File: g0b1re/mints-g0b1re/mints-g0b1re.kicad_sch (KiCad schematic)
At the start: 34 parts, among them J1 Conn_01x08, J3 Conn_01x02, J4 Conn_01x04, J5 Conn_01x04, J6 FTSH-107-01-X-DV-K, J7 Conn_01x04, SW1 SW_Coded_SH-7050, U1 STM32G0B1RETx, U2 TCAN3414DDFR, U5 AP63203WU

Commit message: polishing schematic, add variants, fix some small issues
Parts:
- removed J7: Conn_01x04, Connector_PinHeader_2.54mm:PinHeader_1x04_P2.54mm_Vertical, symbol Connector_Generic:Conn_01x04
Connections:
- net CAN+: now also J4.2 (Pin_2); no longer J5.1 (Pin_1)
- net CAN-: now also J4.3 (Pin_3); no longer J5.4 (Pin_4)
- net GND: now also J4.4 (Pin_4), J5.4 (Pin_4); no longer J4.1 (Pin_1), J4.2 (Pin_2)
- net SPI_nCS: now reaches U1.36 (PA8)
- net CANRX renamed CAN_RXD
- net CAN_RXD: now also U1.25 (PC4); no longer U1.26 (PC5)
- net CANTX renamed CAN_TXD
- net CAN_TXD: now also U1.26 (PC5); no longer U1.25 (PC4)
- net CTRL: no longer names the net of U1.18 (PA1)
- net EXTI renamed ADC_nIRQ
- new net: F1.2, J4.1 (Pin_1), J5.1 (Pin_1)
- no-connect marks 38 -> 39
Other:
- note added: "All capacitors are 0603 X5R 10% and Vw > 50 V unless otherwise marked All resistors are 0603 1% unless otherwise marked"
- note added: "CAN + PWR Plug"
- note added: "Input voltage: 3.8-32V"
- note added: "Output Current: 2A max"
- note added: "Variant 1: ADC"
- note added: "Variant 2: I2C"
- note added: "Variant 3: Outputs"
- note removed: "Add SWO"
- note removed: "Add header for STLINK V3 Mini"
- note removed: "Andrew says to remove blocks and just use whitespace to seperate"
- note removed: "CAN Plug"
- note removed: "Choose good voltae for caps and power/tolerance for resistors and note on schematic (typ "unless otherwise noted")"
- note removed: "Config Option 1: ADC"
- note removed: "Config Option 2: Outputs"
- note removed: "Config Option 3: I2C"
- note removed: "Configuration Instructions For 0-3.3V: R_ADC_TOP: 0 R_ADC_BTM: NP R_ADC_POS: 1k R_ADC_NEG: 1k For 0-33V: R_ADC_TOP: 100k R_ADC_BOT: 11k R_ADC_POS: 0 R_ADC_NEG: 1k For 4-20mA: R_ADC_TOP: 0 R_ADC_BOT: 10 R_ADC_POS: 1k R_ADC_NEG: 1k For higher amps: R_ADC_TOP: 0 R_ADC_BOT: NP R_ADC_POS: 1k R_ADC_NEG: 1k R_SHUNT : shunt"
- note removed: "Decoupling cap? Put it on VCC"
- note removed: "I2C is NOT isolated"
- note removed: "Inculde max input/output specs in label"
- note removed: "Inputs are NOT isolated"
- note removed: "Make this 2 identical 4pin connectors rather than one big so can't plug in wrong spot (each has vbus, gnd, can+, can-)"
- note removed: "One TP to usb+, one to usb-, and one to gnd"
- note removed: "Output Current Limit Each: Max 2.8A continous @ 15C board above ambient Max 6A peak inrush Combined Max 13A continous @ 15C board above ambient"
- note removed: "Outputs are electrically isolated"
- note removed: "Pick exactly one during assembally Use the same option for all channels Do not assemble other options"
- note removed: "Remove net labels if you're not going to use them"
- note removed: "Rename cas CANRX and CANTX"
- note removed: "Route USB D+,D-,Gnd to test point"
- note removed: "Select correct pin names on STM footprint (right click on pin -> choose pin function)"
- note removed: "TODO add expected power supply specs"
- note removed: "TODO check that these are the correct pins"
- note removed: "TODO design change verify support for 4-28v system power input"
- note removed: "TODO name block"
- note removed: "Tie SHDN low"
- note removed: "Upgrade to 50v"
- note removed: "Why no SPI2_NSS?"
- note removed: "add SWDCLK, SWDIO, GND, 3.3v to test header"
- note removed: "add TP and del label"
- note removed: "bit order does not matter on PCB"
- note removed: "probs not right probably cap to gnd"
- note removed: "switch to TCAN3413DDFR"
- note removed: "tie vbat to vdd?"
- title: Mints Scada Hardware -> minTS SCADA Board
- moved on the sheet: C11, C12, C13, C14, C15, C5, C6, C7, C8, C9, D2, D3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

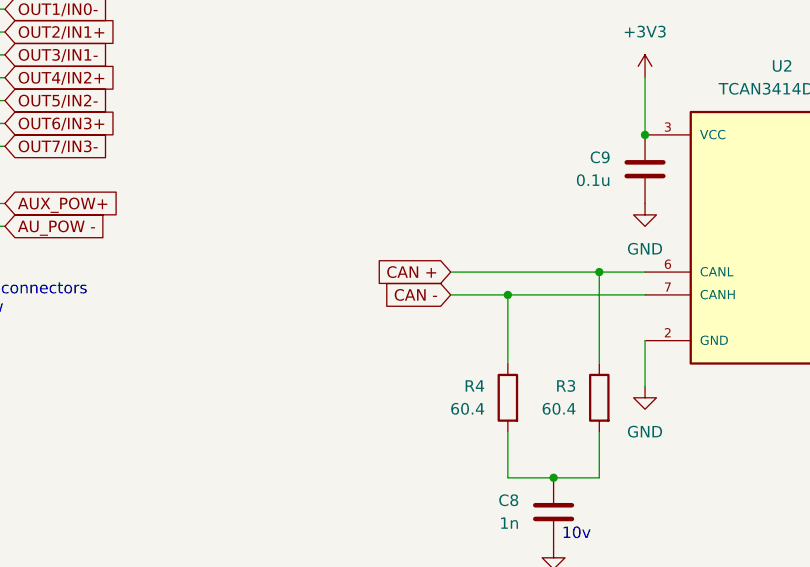
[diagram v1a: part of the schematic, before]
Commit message: board updates 9/2/26
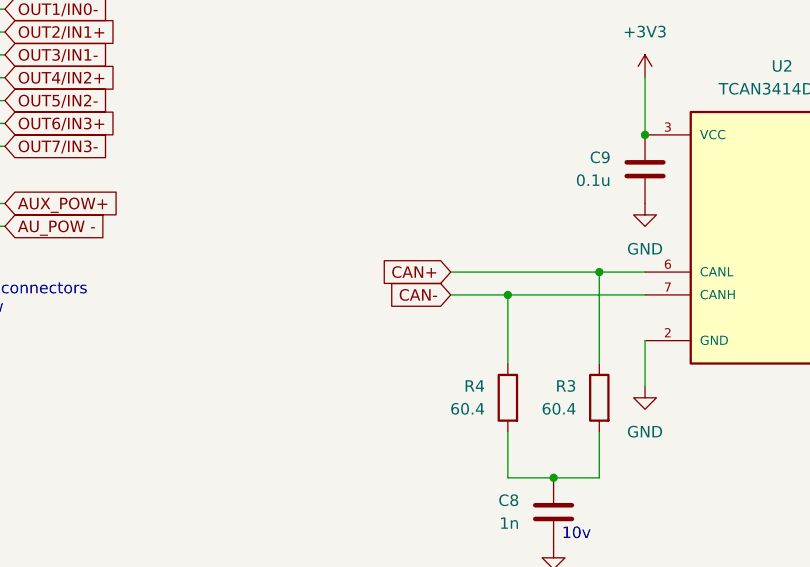
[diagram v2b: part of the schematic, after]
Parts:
- J1: footprint Connector_PinHeader_2.54mm:PinHeader_1x08_P2.54mm_Vertical -> Connector_Phoenix_MSTB:PhoenixContact_MSTBA_2,5_8-G-5,08_1x08_P5.08mm_Horizontal
- J3: footprint TerminalBlock_Phoenix:TerminalBlock_Phoenix_MKDS-1,5-2-5.08_1x02_P5.08mm_Horizontal -> Connector_Phoenix_MSTB:PhoenixContact_MSTBA_2,5_2-G-5,08_1x02_P5.08mm_Horizontal
- J4, J5: footprint Connector_PinHeader_2.54mm:PinHeader_1x04_P2.54mm_Vertical -> Connector_Phoenix_MSTB:PhoenixContact_MSTBA_2,5_4-G-5,08_1x04_P5.08mm_Horizontal
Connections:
- net CAN + is gone; now on net CAN+: R3.1, U2.6 (CANL)
- net CAN - is gone; now on net CAN-: R4.1, U2.7 (CANH)
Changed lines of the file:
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@@
 		)
 	)
-	(global_label "CAN +"
+	(global_label "CAN+"
 		(shape input)
 		(at 120.65 132.08 180)
@@
 		)
 		(property "Intersheetrefs" "${INTERSHEET_REFS}"
-			(at 111.4357 132.08 0)
+			(at 112.4033 132.08 0)
 			(hide yes)
 			(show_name no)
@@
 		)
 	)
-	(global_label "CAN -"
+	(global_label "CAN-"
 		(shape input)
 		(at 120.65 134.62 180)
@@
 		)
 		(property "Intersheetrefs" "${INTERSHEET_REFS}"
-			(at 111.4357 134.62 0)
+			(at 112.4033 134.62 0)
 			(hide yes)
 			(show_name no)
@@
 			)
 		)
-		(property "Footprint" "TerminalBlock_Phoenix:TerminalBlock_Phoenix_MKDS-1,5-2-5.08_1x02_P5.08mm_Horizontal"
+		(property "Footprint" "Connector_Phoenix_MSTB:PhoenixContact_MSTBA_2,5_2-G-5,08_1x02_P5.08mm_Horizontal"
 			(at 57.15 124.46 0)
 			(hide yes)
@@
 			)
 		)
-		(property "Footprint" "Connector_PinHeader_2.54mm:PinHeader_1x08_P2.54mm_Vertical"
+		(property "Footprint" "Connector_Phoenix_MSTB:PhoenixContact_MSTBA_2,5_8-G-5,08_1x08_P5.08mm_Horizontal"
 			(at 57.15 107.95 0)
 			(hide yes)
@@
 			)
 		)
-		(property "Footprint" "Connector_PinHeader_2.54mm:PinHeader_1x04_P2.54mm_Vertical"
+		(property "Footprint" "Connector_Phoenix_MSTB:PhoenixContact_MSTBA_2,5_4-G-5,08_1x04_P5.08mm_Horizontal"
 			(at 57.15 73.66 0)
 			(hide yes)
@@
 			)
 		)
-		(property "Footprint" "Connector_PinHeader_2.54mm:PinHeader_1x04_P2.54mm_Vertical"
+		(property "Footprint" "Connector_Phoenix_MSTB:PhoenixContact_MSTBA_2,5_4-G-5,08_1x04_P5.08mm_Horizontal"
 			(at 57.15 54.61 0)
 			(hide yes)
